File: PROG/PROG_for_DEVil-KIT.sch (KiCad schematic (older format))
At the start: 27 parts, among them J1 POWER, J2 PROG, Q1 BSS138LT1G, Q2 BSS138LT1G, Q3 BSS138LT1G, Q4 BSS138LT1G, U1 AMS1117-3.3

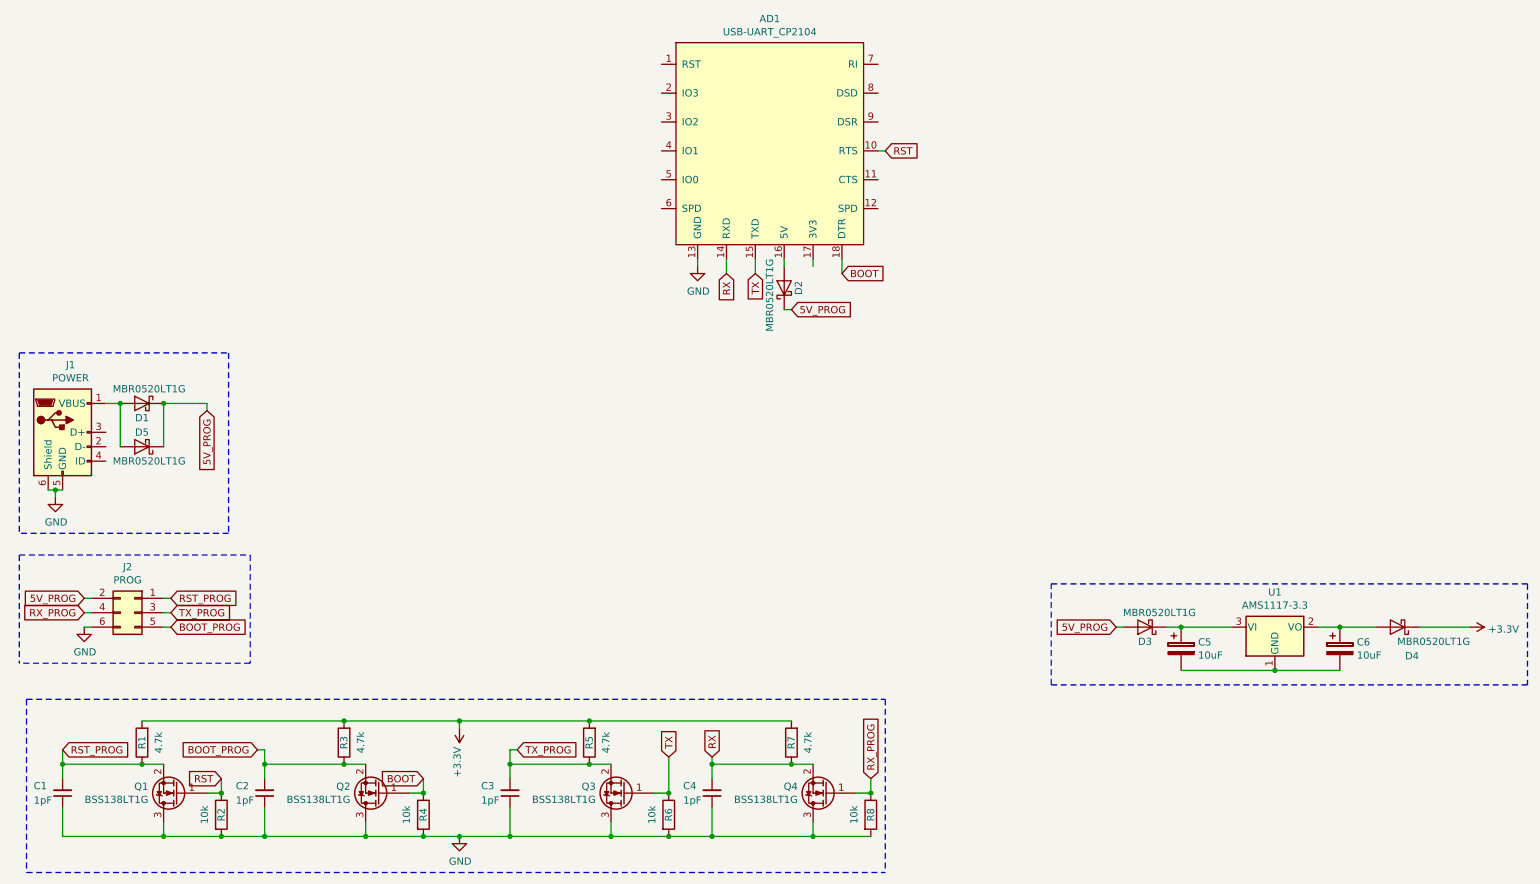
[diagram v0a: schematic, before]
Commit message: Add files via upload
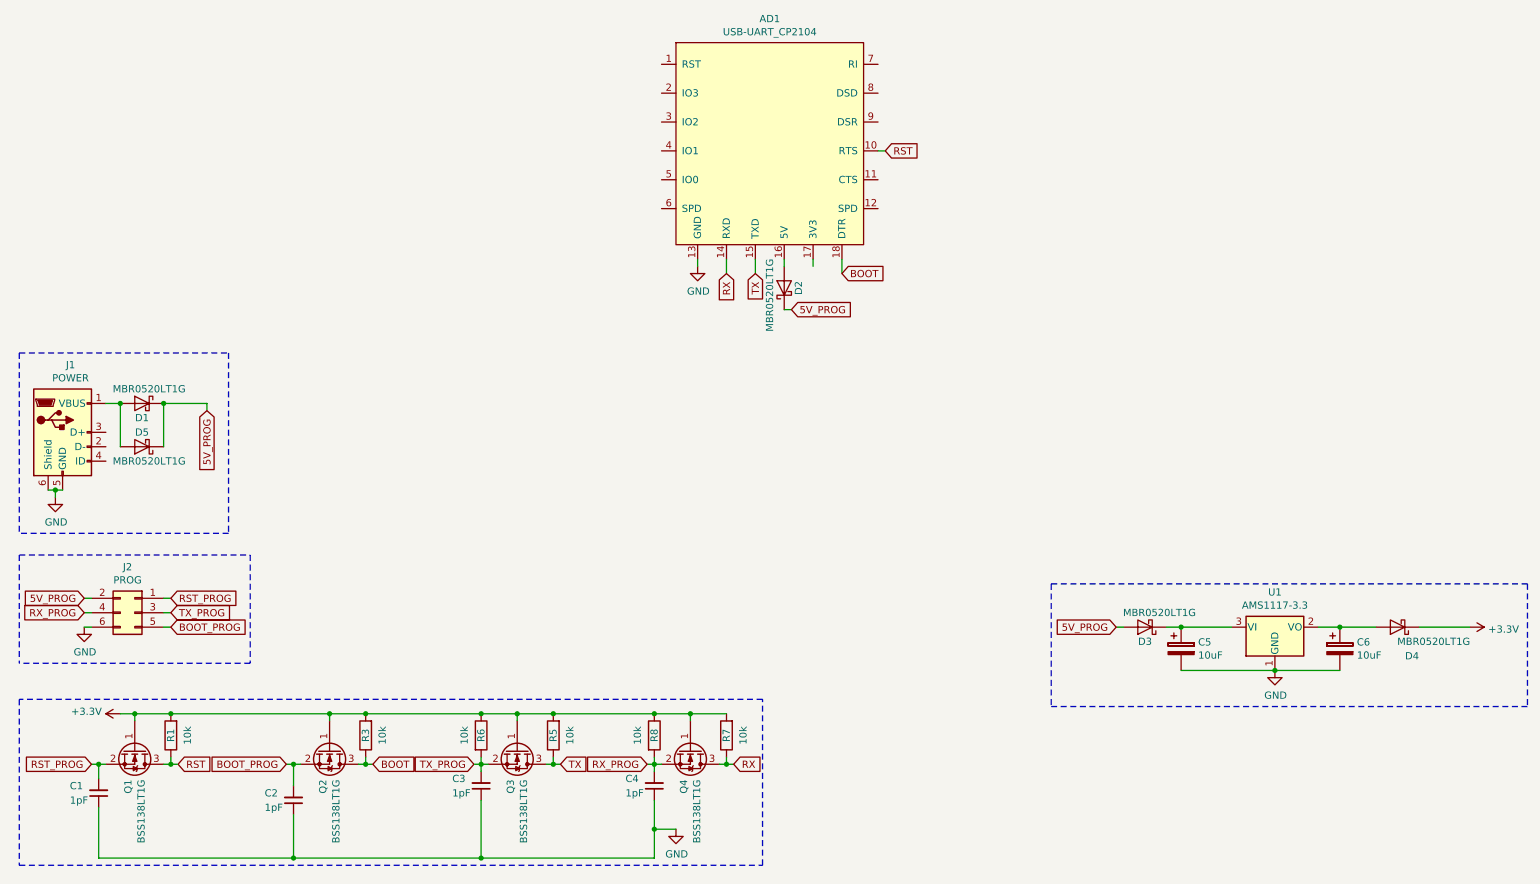
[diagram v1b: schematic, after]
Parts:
- removed R2, R4: 10k, Resistor_SMD:R_0603_1608Metric_Pad1.05x0.95mm_HandSolder, symbol Device:R
- R1, R3, R5, R7: value 4.7k -> 10k
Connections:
- net +3V3: now also Q1.1 (G), Q2.1 (G), Q3.1 (G), Q4.1 (G), R6.1, R8.1
- net BOOT: now also Q2.3 (D), R3.1; no longer Q2.1 (G)
- net BOOT_PROG: no longer R3.1
- net GND: now also C5.2, C6.2, U1.1 (GND); no longer Q1.3 (D), Q2.3 (D), Q3.3 (D), Q4.3 (D), R6.2, R8.2
- net RST: now also Q1.3 (D), R1.1; no longer Q1.1 (G)
- net RST_PROG: no longer R1.1
- net RX: now also Q4.3 (D); no longer C4.2, Q4.2 (S)
- net RX_PROG: now also C4.2, Q4.2 (S), R8.2; no longer Q4.1 (G), R8.1
- net TX: now also Q3.3 (D), R5.1; no longer Q3.1 (G), R6.1
- net TX_PROG: now also R6.2; no longer R5.1
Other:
- moved on the sheet: C1, C2, C3, C4, Q1, Q2, Q3, Q4, R1, R3, R5, R6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
